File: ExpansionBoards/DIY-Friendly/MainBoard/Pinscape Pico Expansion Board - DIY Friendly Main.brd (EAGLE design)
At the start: 160 x 100 mm, 114 parts, among them IC1 UCC27524P, IC10 ULN2803A, IC11 SN74HC165N, IC12 SN74HC165N, IC13 SN74HC74NE4, IC14 PC827, IC15 S-80833CLY, IC16 SN74HC165N, IC18 SN74HC165N, IC2 UCC27524P, IC3 UCC27524P, IC4 UCC27524P, IC5 UCC27524P, IC6 UCC27524P, IC7 ULN2803A, IC8 ULN2803A, IC9 ULN2803A, J1 30316-6002HB, J10 215079-4, J11 640454-2, J13 640445-2, J2 640445-6, J3 640445-5, J4 640445-9, J5 1-640456-0, J6 1-640456-0, J7 1-640456-0, J8 1-640456-0, J9 30308-6002HB, Q1 FDPF085N10A, Q10 FDPF085N10A, Q11 FDPF085N10A, Q12 FDPF085N10A, Q13 BC337-25, Q15 2N5195G, Q16 2N2222A, Q2 FDPF085N10A, Q3 FDPF085N10A, Q4 FDPF085N10A, Q5 FDPF085N10A, Q6 FDPF085N10A, Q7 FDPF085N10A, Q8 FDPF085N10A, Q9 FDPF085N10A

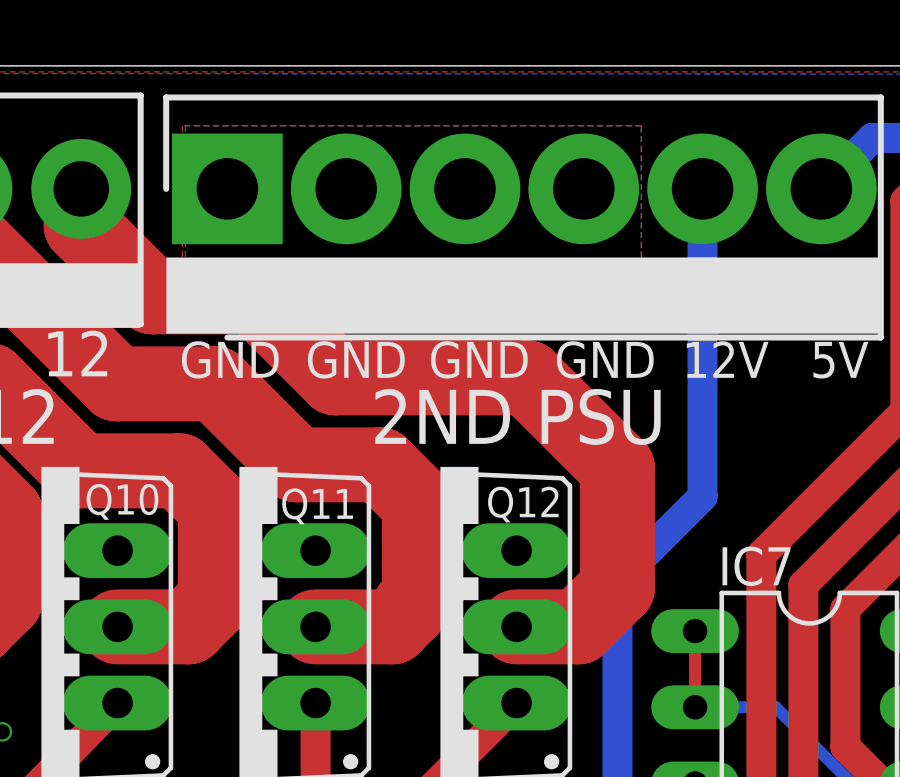
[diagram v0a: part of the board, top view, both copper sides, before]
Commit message: add logo image
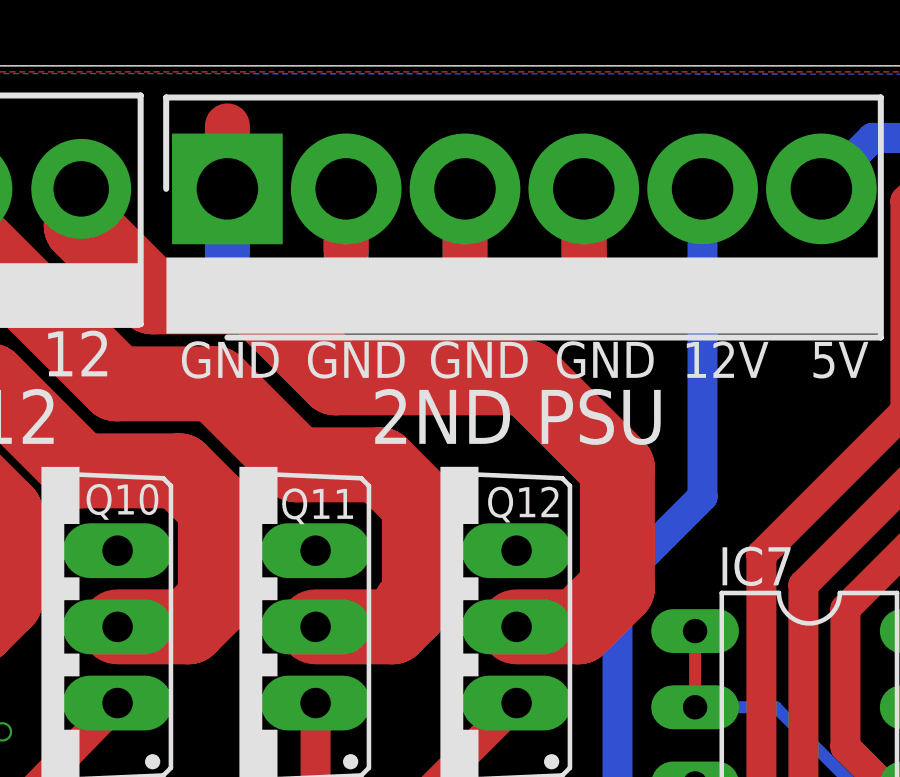
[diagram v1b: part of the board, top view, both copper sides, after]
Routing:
- net GND: track 0.00 -> 17.6 mm
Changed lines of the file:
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@@
 <contactref element="D4" pad="C"/>
 <contactref element="R31" pad="1"/>
-<polygon width="1" layer="1" thermals="no">
-<vertex x="94.8" y="93.3"/>
-<vertex x="110.1" y="93.3"/>
-<vertex x="110.1" y="98"/>
-<vertex x="94.8" y="98"/>
-</polygon>
-<polygon width="1" layer="16" thermals="no">
-<vertex x="94.9" y="93.3"/>
-<vertex x="110.1" y="93.3"/>
-<vertex x="110.1" y="98"/>
-<vertex x="94.9" y="98"/>
-</polygon>
 <contactref element="J2" pad="1"/>
 <contactref element="J2" pad="2"/>
@@
 <vertex x="147.2" y="61.5"/>
 </polygon>
+<wire x1="96.3" y1="95.9" x2="96.3" y2="93.7" width="1.5" layer="16"/>
+<wire x1="100.26" y1="95.9" x2="100.26" y2="93.64" width="1.5" layer="16"/>
+<wire x1="104.22" y1="95.9" x2="104.22" y2="93.68" width="1.5" layer="16"/>
+<wire x1="108.18" y1="95.9" x2="108.18" y2="93.62" width="1.5" layer="16"/>
+<wire x1="96.3" y1="95.9" x2="96.3" y2="98" width="1.5" layer="1"/>
+<wire x1="100.26" y1="95.9" x2="100.26" y2="93.84" width="1.5" layer="1"/>
+<wire x1="104.22" y1="95.9" x2="104.22" y2="93.72" width="1.5" layer="1"/>
+<wire x1="108.18" y1="95.9" x2="108.2" y2="93.6" width="1.5" layer="1"/>
 </signal>
 <signal name="SDA">
@@
 <wire x1="109.3" y1="69.4" x2="109.3" y2="82.8" width="1" layer="16"/>
 <wire x1="107.93" y1="68.03" x2="107.3" y2="68.03" width="1" layer="16"/>
-<wire x1="110.284" y1="83.784" x2="109.6" y2="83.1" width="1" layer="16"/>
 <contactref element="J2" pad="5"/>
-<wire x1="109.6" y1="83.1" x2="109.3" y2="82.8" width="1" layer="16"/>
 <wire x1="112.14" y1="95.9" x2="112.14" y2="85.64" width="1" layer="16"/>
-<wire x1="112.14" y1="85.64" x2="110.284" y2="83.784" width="1" layer="16"/>
+<wire x1="112.14" y1="85.64" x2="109.3" y2="82.8" width="1" layer="16"/>
 </signal>
 <signal name="OUTCTL2">
